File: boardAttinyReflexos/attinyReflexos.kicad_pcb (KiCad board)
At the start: 2 copper layers, 43.2 x 43.2 mm, 17 parts, among them J1 Conn_01x06_Female, SW1 SW_DPST_x2, SW2 SW_DIP_x01, U1 ATTINY85-20PU

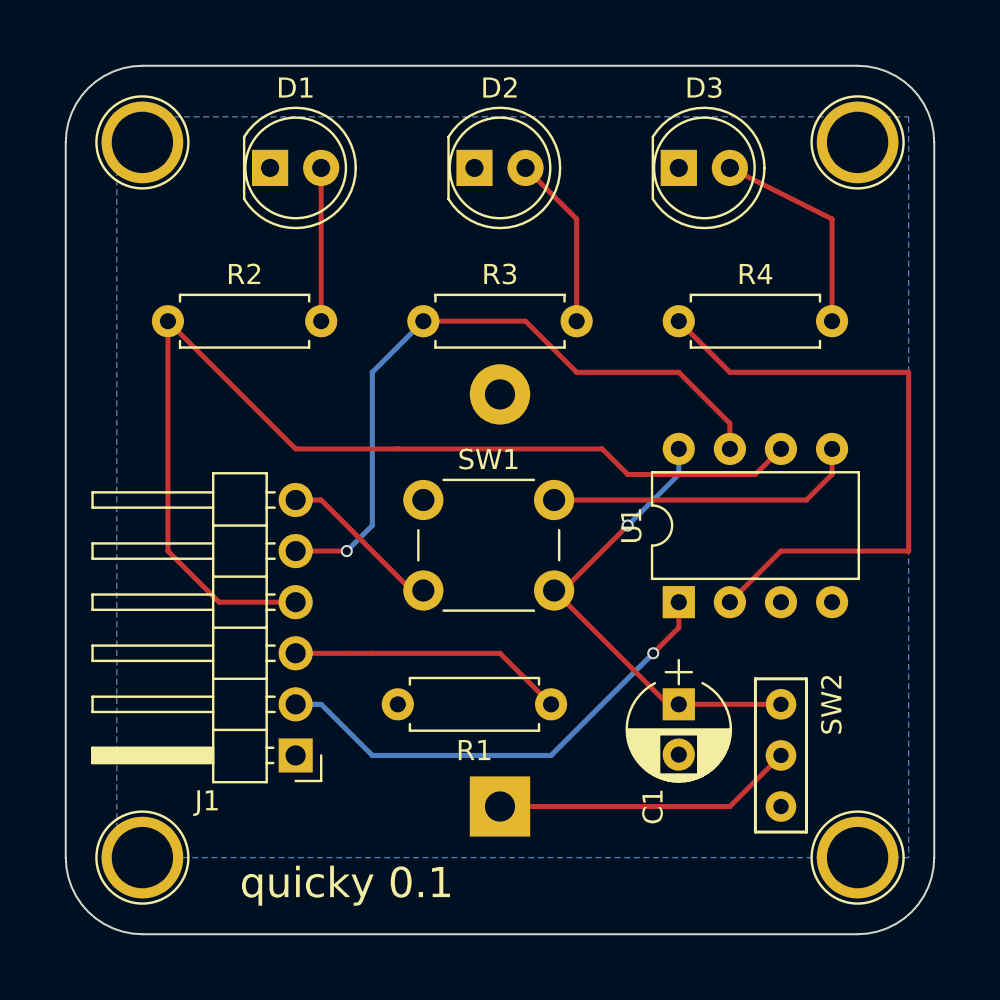
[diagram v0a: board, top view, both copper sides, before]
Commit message: corrixido erro
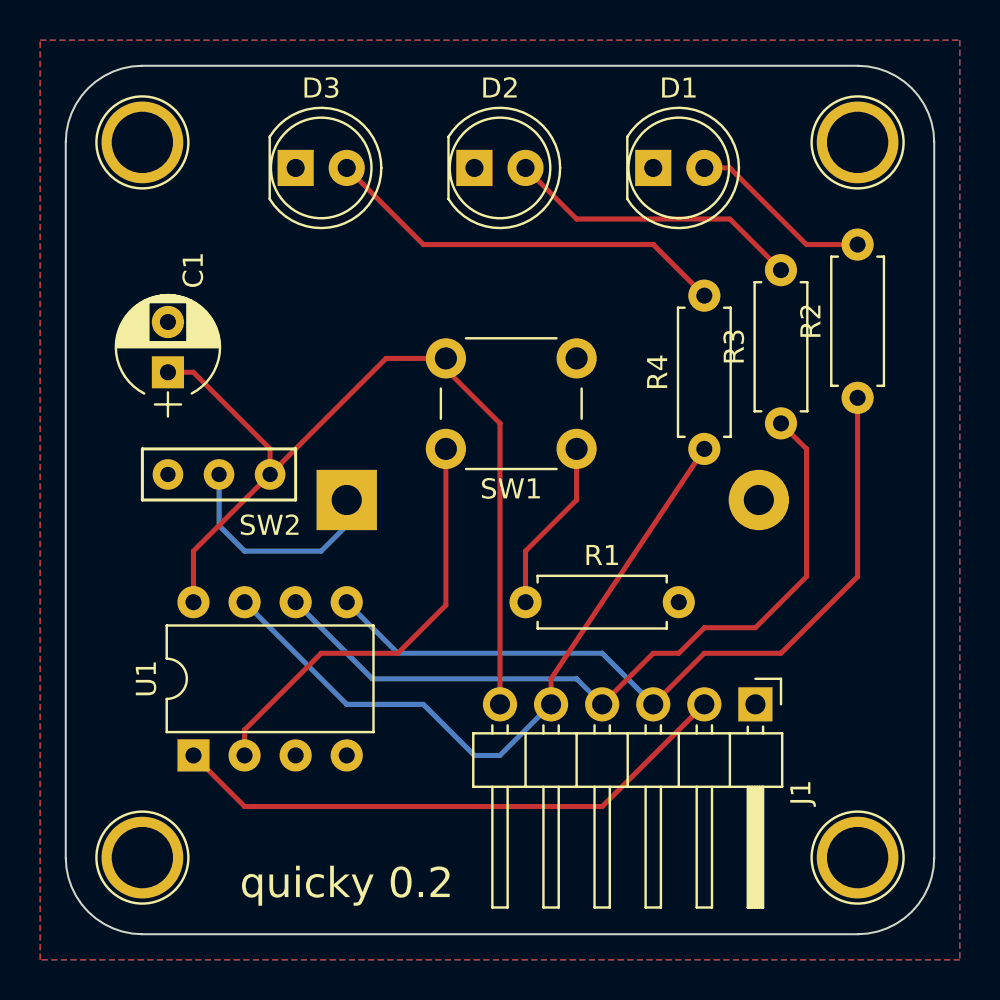
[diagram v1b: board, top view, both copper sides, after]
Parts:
- moved R2 34.5 mm to (174.0, 106.7), turned to 90 degrees
- moved SW2 31.2 mm to (142.2, 110.5), turned to 180 degrees
- moved C1 30.3 mm to (139.7, 105.4), turned to 90 degrees
- moved U1 25.3 mm to (141.0, 124.5)
- moved J1 23.0 mm to (168.9, 121.9), turned to 270 degrees
- moved D1 19.1 mm to (163.8, 95.2)
- moved D3 19.0 mm to (146.1, 95.2)
- moved R3 18.5 mm to (170.2, 108.0), turned to 90 degrees
- moved BT1 17.0 mm to (148.6, 111.8), turned to 0 degrees
- moved SW1 8.03 mm to (160.0, 109.2), turned to 180 degrees
- moved R4 6.48 mm to (166.4, 109.2), turned to 90 degrees
- moved R1 5.24 mm to (157.5, 116.8), turned to 0 degrees
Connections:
- R1 pad 1: Net-(J1-Pad3) -> Net-(R1-Pad1)
- R2 pad 1: Net-(J1-Pad4) -> Net-(J1-Pad3)
- R3 pad 1: Net-(J1-Pad5) -> Net-(J1-Pad4)
- R4 pad 1: Net-(R4-Pad1) -> Net-(J1-Pad5)
- SW1 pad 1: Net-(J1-Pad3) -> Net-(R1-Pad1)
- U1 pad 2: Net-(R4-Pad1) -> Net-(R1-Pad1)
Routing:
- net Net-(R4-Pad1): track 31.3 -> 0.00 mm
- net Net-(R1-Pad1): track 0.00 -> 30.3 mm
- net Net-(J1-Pad4): track 53.0 -> 38.3 mm
- net VCC: track 31.7 -> 45.3 mm, vias 1 -> 0
- net Net-(J1-Pad3): track 29.4 -> 39.0 mm
- net Net-(D3-Pad2): track 10.8 -> 20.4 mm
- net Net-(D2-Pad2): track 8.67 -> 14.8 mm
- net Net-(J1-Pad2): track 24.0 -> 28.6 mm, vias 1 -> 0
- net Net-(BT1-Pad1): track 15.0 -> 11.2 mm
- net Net-(D1-Pad2): track 7.62 -> 9.20 mm
- net Net-(J1-Pad5): track 34.2 -> 34.5 mm, vias 1 -> 0
- added copper zone on F.Cu, net GND
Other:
- board text added: "quicky 0.2"
- board text removed: "quicky 0.1"
